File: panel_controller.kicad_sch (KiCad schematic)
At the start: 9 parts, among them J1 SBH11-PBPC-D08-ST-BK, J2 215297-6, J3 Screw_Terminal_01x03, J4 Screw_Terminal_01x02, U1 ESP32-DEVKIT-V1

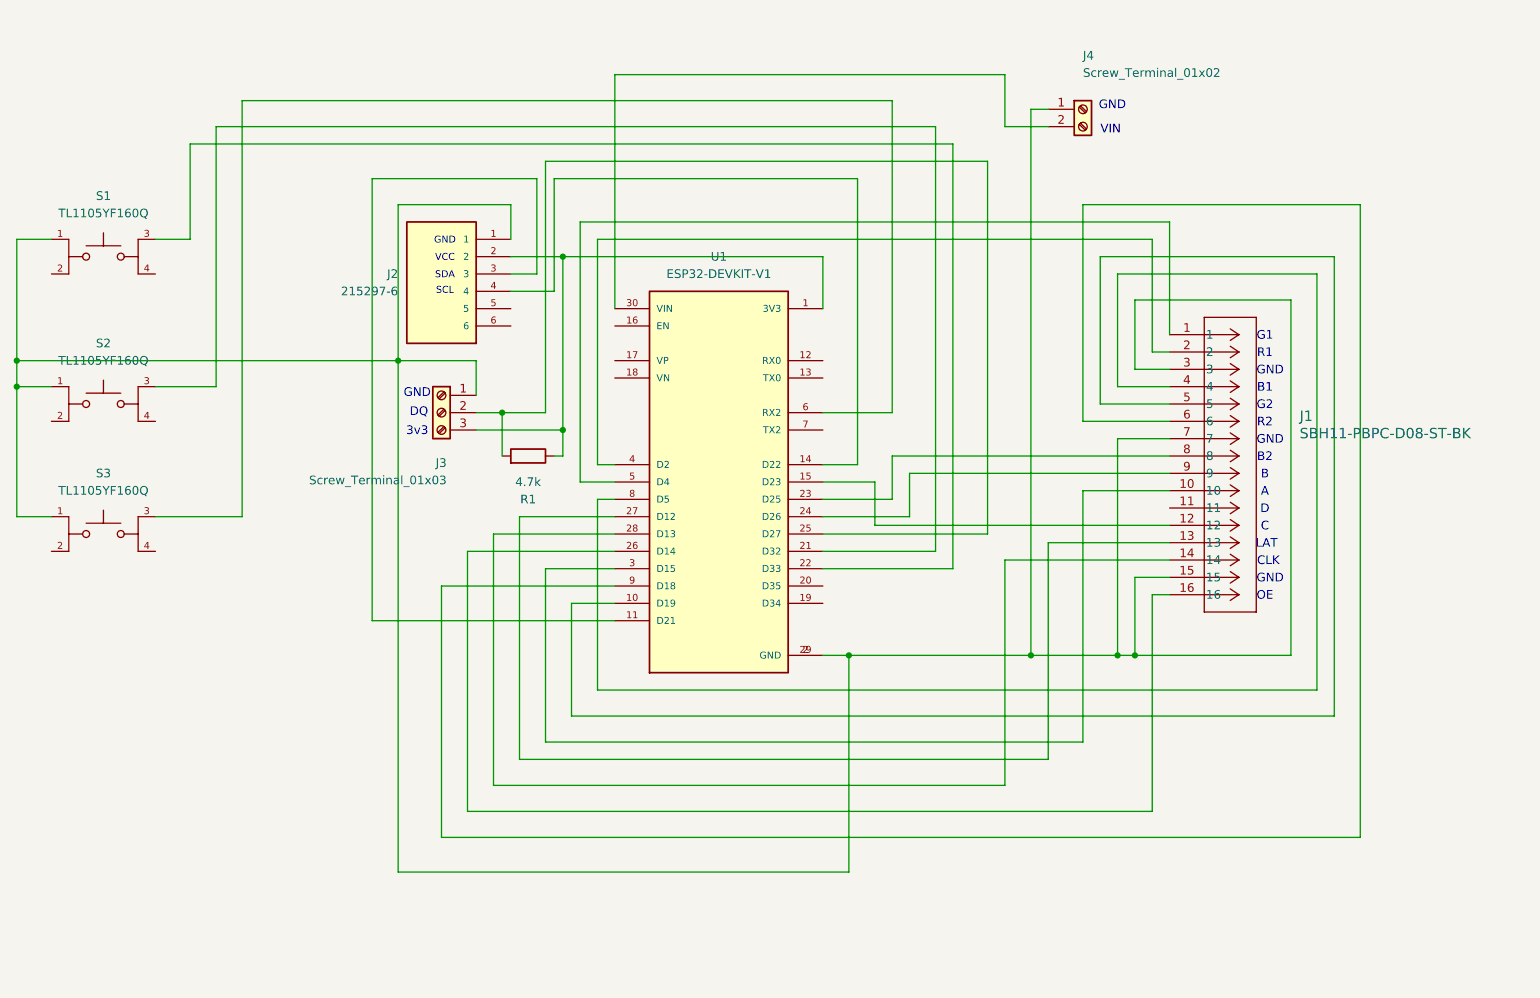
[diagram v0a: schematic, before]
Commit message: pcb clock v1.2
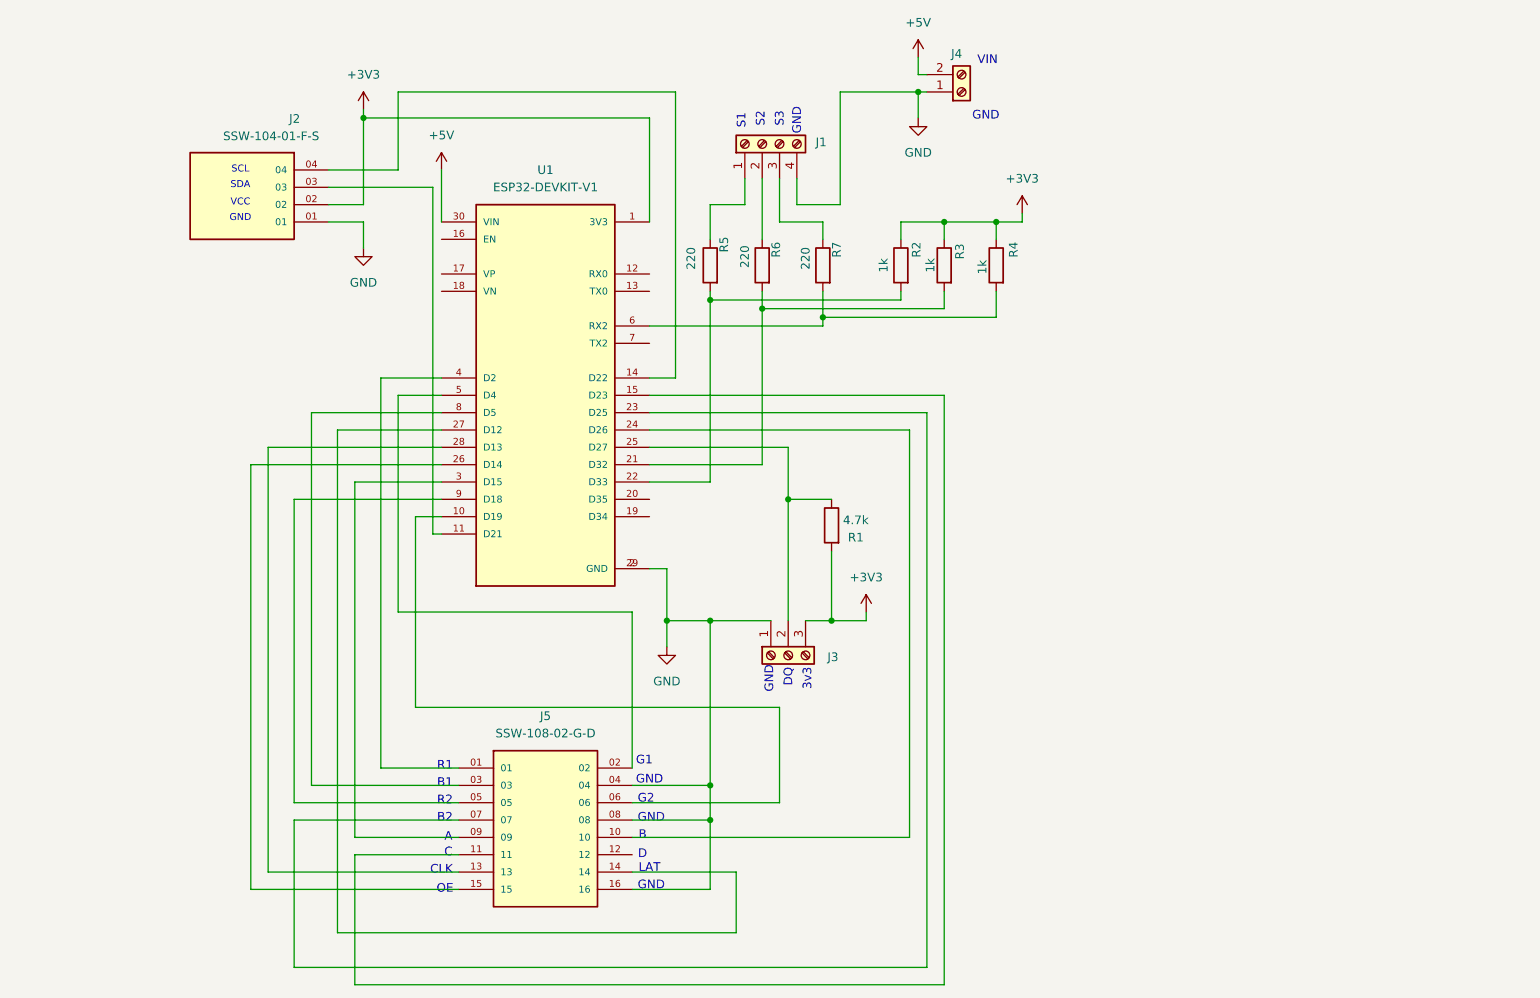
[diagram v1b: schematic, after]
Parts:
- removed J1: SBH11-PBPC-D08-ST-BK, CONN16_SBH11-PBPC-D08-ST-BK_SUL, symbol 2025-08-25_13-41-09:SBH11-PBPC-D08-ST-BK
- removed J2: 215297-6, 215297_6:TE_215297-6, symbol 215297-6:215297-6
- removed S1, S2, S3: TL1105YF160Q, TL1105YF160Q:SW_TL1105YF160Q, symbol TL1105YF160Q:TL1105YF160Q
- added J1: Screw_Terminal_01x04, TerminalBlock:TerminalBlock_Altech_AK300-4_P5.00mm, symbol Connector:Screw_Terminal_01x04
- added J2: SSW-104-01-F-S, SSW-104-01-F-S:SAMTEC_SSW-104-01-F-S-RTC, symbol SSW-104-01-F-S:SSW-104-01-F-S
- added J5: SSW-108-02-G-D, SSW-108-02-G-D:SAMTEC_SSW-108-02-G-D, symbol SSW-108-02-G-D:SSW-108-02-G-D
- added R2, R3, R4: 1k, Resistor_THT:R_Axial_DIN0204_L3.6mm_D1.6mm_P5.08mm_Horizontal, symbol Device:R
- added R5, R6, R7: 220, Resistor_THT:R_Axial_DIN0204_L3.6mm_D1.6mm_P5.08mm_Horizontal, symbol Device:R
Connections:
- net GND: now reaches J3.1 (Pin_1), J4.1 (Pin_1), U1.2 (GND), U1.29 (GND)
- net GND: now also J1.4 (Pin_4), J2.01, J5.04, J5.08, J5.16
- net at J3.2 (Pin_2), U1.25 (D27): now also R1.1; no longer R1.2
- net +3V3: now reaches J3.3 (Pin_3), U1.1 (3V3)
- net +3V3: now also R1.2, J2.02, R2.1, R3.1, R4.1; no longer R1.1
- net at U1.5 (D4): now also J5.02
- net at U1.3 (D15): now also J5.09
- net at U1.15 (D23): now also J5.11
- net at U1.27 (D12): now also J5.14
- net at U1.28 (D13): now also J5.13
- net at U1.26 (D14): now also J5.15
- net at U1.4 (D2): now also J5.01
- net at U1.8 (D5): now also J5.03
- net at U1.10 (D19): now also J5.06
- net at U1.9 (D18): now also J5.05
- net at U1.23 (D25): now also J5.07
- net at U1.24 (D26): now also J5.10
- net at U1.22 (D33): now also R2.2, R5.2
- net at U1.11 (D21): now also J2.03
- net at U1.14 (D22): now also J2.04
- net at U1.21 (D32): now also R3.2, R6.2
- net +5V: now reaches J4.2 (Pin_2), U1.30 (VIN)
- net at U1.6 (RX2): now also R4.2, R7.2
- new net: J1.1 (Pin_1), R5.1
- new net: J1.2 (Pin_2), R6.1
- new net: J1.3 (Pin_3), R7.1
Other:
- note added: "S1"
- note added: "S2"
- note added: "S3"
- moved on the sheet: J3, J4, R1, U1
